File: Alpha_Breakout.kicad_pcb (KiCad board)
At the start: 4 copper layers, 66.7 x 74.4 mm, 161 parts, among them IC1 LM66200DRLR, J10 Conn_01x03, J11 Conn_01x03, J12 Conn_01x03, J14 Conn_01x03, J15 Conn_01x03, J16 Conn_01x03, J18 Conn_01x02, J19 Conn_01x02, J2 USB_C_Receptacle_USB2.0_16P, J20 Conn_01x02, J21 Conn_01x02, J22 Conn_01x02, J23 Conn_01x02, J24 Conn_01x04, J25 Conn_01x02, J26 Conn_01x02, J27 Conn_01x02, J28 Conn_01x02, J29 Conn_01x02, J3 Conn_01x03, J30 Conn_01x04, J31 Conn_01x02, J33 Conn_01x02, J34 Conn_01x02, J35 Conn_02x06_Odd_Even, J36 Conn_01x02, J4 Conn_01x03, J5 Conn_01x03, J7 Conn_01x03, J8 Conn_01x03, J9 Conn_01x03, Q1 CSD13381F4, Q2 CSD13381F4, Q3 CSD13381F4, Q4 CSD13381F4, Q5 SSM3J328R, Q6 L2N7002SLLT1G, SW1 SW_Push, SW2 SW_Push, U1 STM32F103C8Tx, U10 LP2985-3.3, U11 SP3485EN, U12 ADS1231ID, U13 TCA9517ADGK, U2 CH340N, U3 ADS7828, U4 ADS7828, U5 MAX31856, U6 MAX31856, U7 MAX31856, U8 MAX31856, U9 AP63203WU

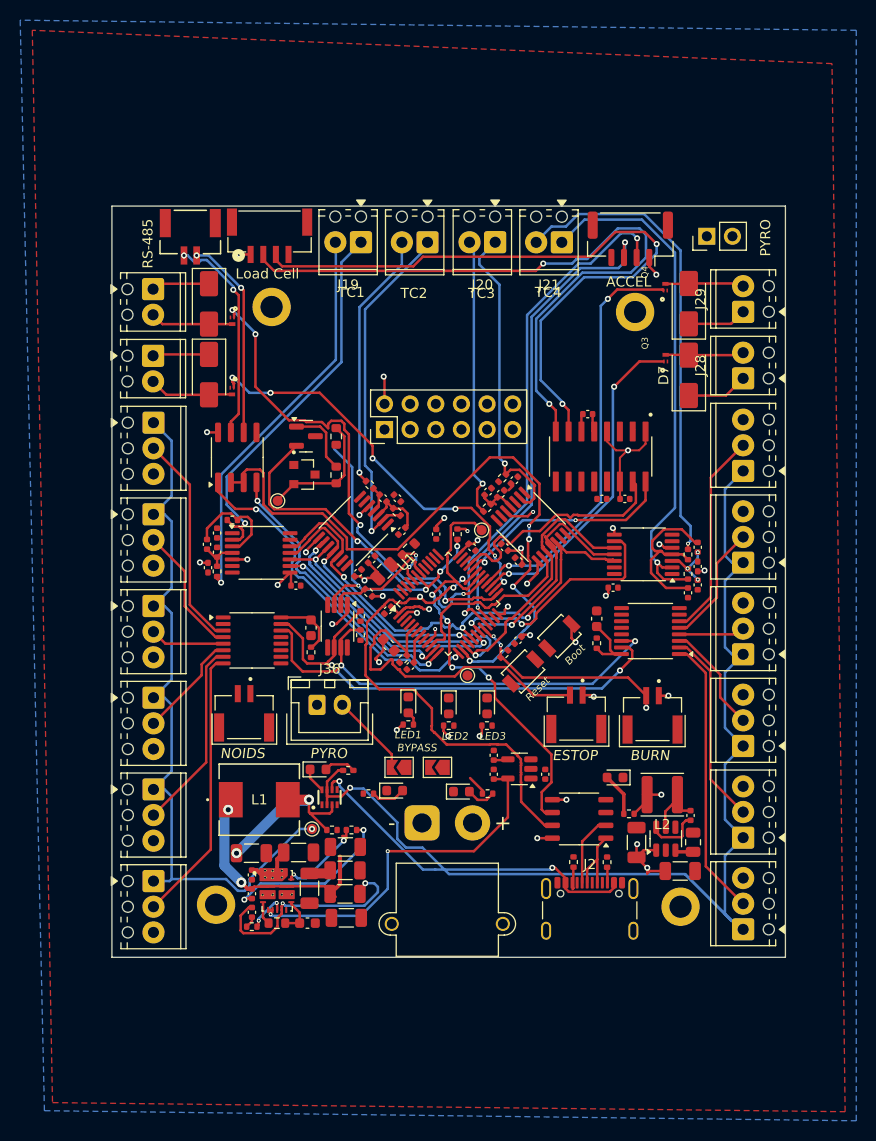
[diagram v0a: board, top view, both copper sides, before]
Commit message: ⚡️⚙️🐘😂
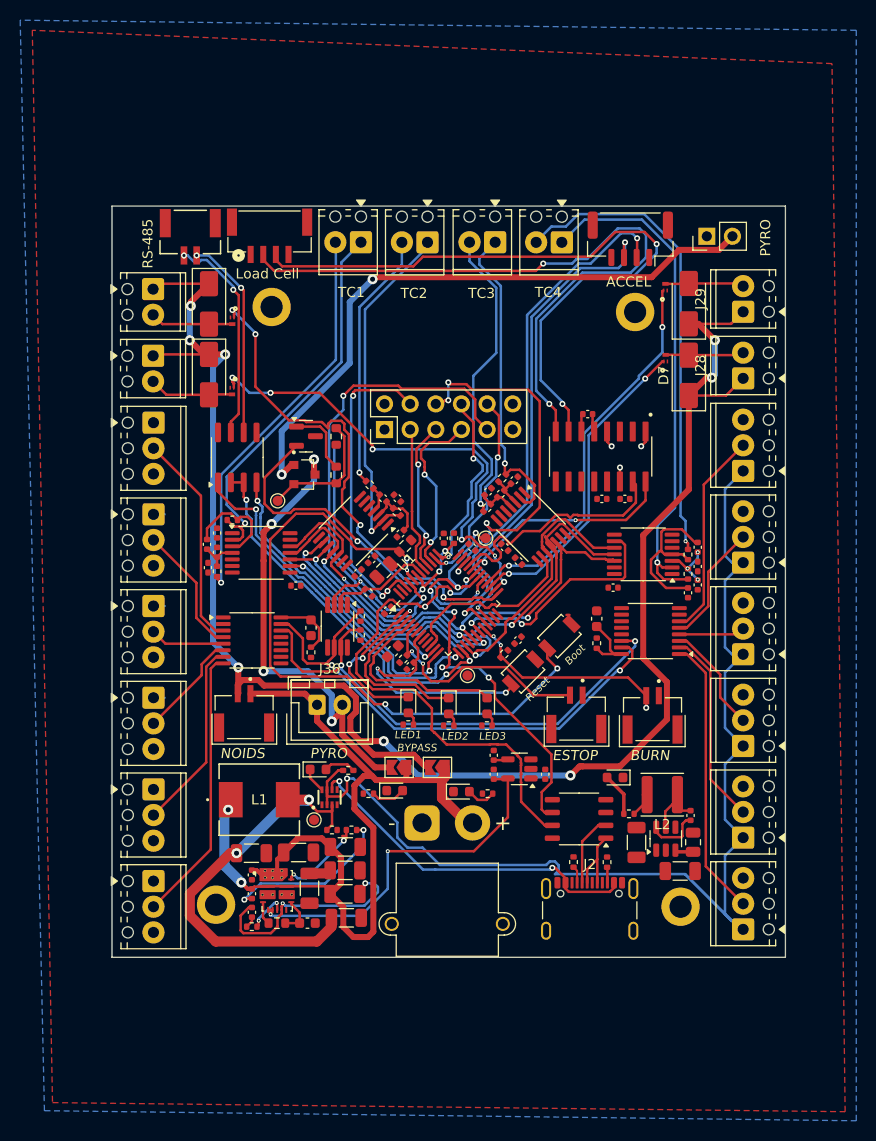
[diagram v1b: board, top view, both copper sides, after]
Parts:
- moved TP4 0.92 mm to (135.1, 123.1)
- moved TP1 0.89 mm to (152.1, 95.2)
- moved C2 0.85 mm to (147.9, 95.2)
- moved C7 0.73 mm to (142.9, 106.4), turned to 45 degrees
- moved R2 0.54 mm to (148.9, 95.2)
- moved R3 0.49 mm to (144.1, 96.0)
- moved C12 0.28 mm to (143.7, 94.7)
- moved C5 0.11 mm to (142.0, 98.4)
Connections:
- J22 pad 1: +BATT -> GND
- J22 pad 2: GND -> +BATT
- J35 pad 3: /Breakout/PB3 -> /Breakout/PB5
- J35 pad 7: /Breakout/PB5 -> /Breakout/PB3
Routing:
- net SW_PWR: track 23.5 -> 174.6 mm, vias 0 -> 8
- net +3.3V: track 85.8 -> 7.88 mm, vias 38 -> 3
- net +5V: track 189.6 -> 120.5 mm, vias 3 -> 1
- net +BATT: track 6.20 -> 71.9 mm
- net Net-(J34-Pin_2): track 0.00 -> 62.1 mm, vias 0 -> 2
- net Net-(U1-BOOT0): track 4.39 -> 66.3 mm, vias 2 -> 4
- net /Breakout/PB8: track 0.00 -> 49.3 mm, vias 0 -> 2
- net /Breakout/PA13: track 0.00 -> 37.6 mm, vias 0 -> 4
- net PYRO_PWR: track 8.23 -> 45.7 mm, vias 0 -> 4
- net /Breakout/PB9: track 0.00 -> 31.1 mm, vias 0 -> 3
- net /RS-485/DIR_RS485: track 67.8 -> 38.1 mm, vias 4 -> 3
- net BATT_V+: track 20.8 -> 45.6 mm
- net Net-(U1-NRST): track 2.97 -> 23.6 mm, vias 0 -> 2
- net /Breakout/PA15: track 0.00 -> 20.3 mm, vias 0 -> 2
- net Net-(D11-K): track 0.00 -> 19.4 mm
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- added copper zone on In2.Cu, net +5V

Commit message: Routed Ground, except for one pad
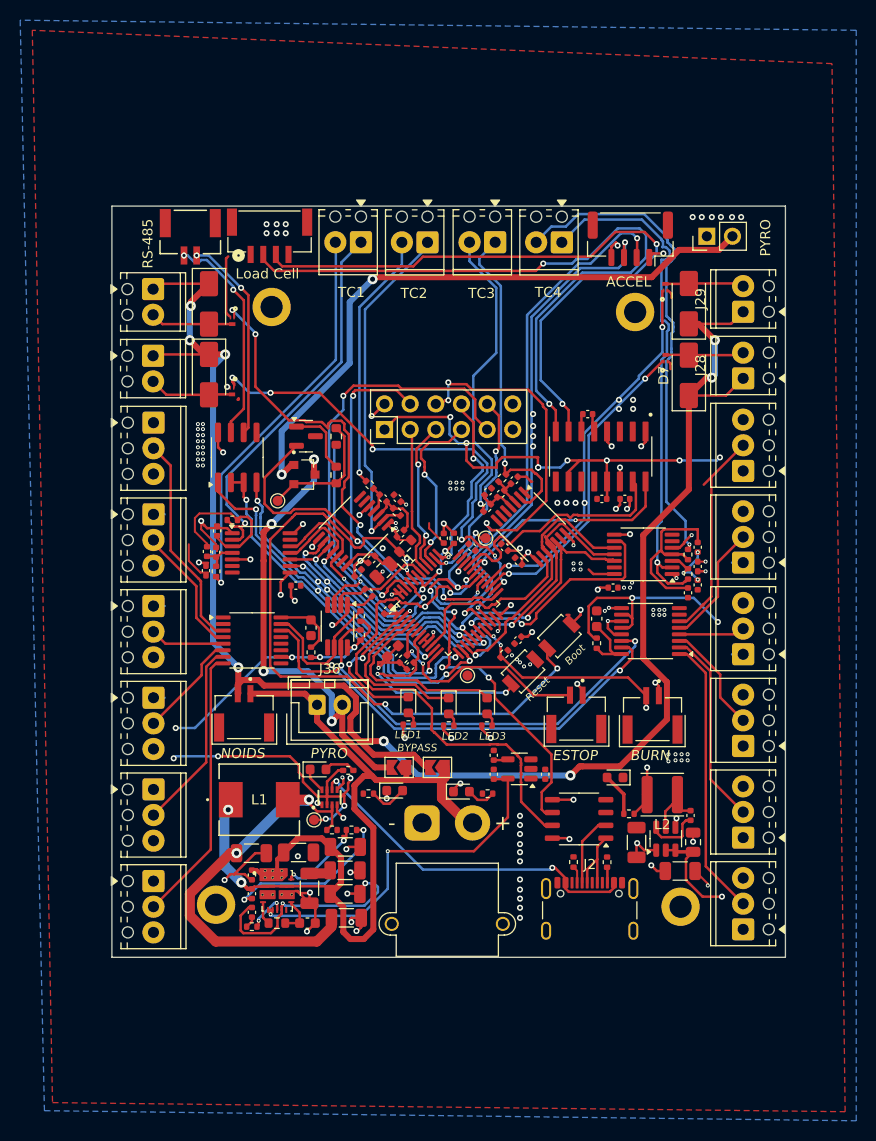
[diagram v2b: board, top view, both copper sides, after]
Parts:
- moved C15 0.71 mm to (124.5, 96.5)
- moved C17 0.36 mm to (124.4, 98.4)
- moved C13 0.21 mm to (125.5, 94.5)
- moved R8 0.10 mm to (125.4, 98.5)
- moved C11 0.10 mm to (125.4, 96.6)
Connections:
- C16 pad 2: +3.3V -> GND
- C17 pad 2: +3.3V -> GND
- C18 pad 1: +3.3V -> GND
- C19 pad 1: +3.3V -> GND
- C2 pad 1: +3.3V -> GND
- C26 pad 2: +3.3V -> GND
- C27 pad 2: +3.3V -> GND
- C28 pad 1: +3.3V -> GND
- C29 pad 1: +3.3V -> GND
- C3 pad 1: +3.3V -> GND
- C30 pad 1: FB -> GND
- C36 pad 1: +3.3V -> GND
- C41 pad 1: +3.3V -> GND
- C5 pad 1: +3.3V -> GND
- C50 pad 2: +3.3V -> GND
- C6 pad 1: +3.3V -> GND
- C7 pad 1: +3.3V -> GND
- J24 pad 1: +3.3V -> GND
- J24 pad 3: /Accelerometer/ACC_SCL -> GND
- J31 pad 1: +3.3V -> GND
- J33 pad 1: +3.3V -> GND
- J35 pad 2: +3.3V -> GND
- L2 pad 2: +3.3V -> GND
- PS1 pad 8: FB -> GND
- Q3 pad 1: /Solenoids/S3 -> GND
- Q4 pad 1: /Solenoids/S4 -> GND
- R1 pad 1: +3.3V -> GND
- R18 pad 1: +3.3V -> GND
- R2 pad 1: +3.3V -> GND
- R28 pad 1: +3.3V -> GND
- R29 pad 1: +3.3V -> GND
- R30 pad 1: +3.3V -> GND
- SW2 pad 1: +3.3V -> GND
- U1 pad 1: +3.3V -> GND
- U1 pad 11: /stm32f1/TC3_CS -> GND
- U1 pad 12: /RS-485/TX_RS485 -> GND
- U1 pad 13: /RS-485/RX_RS485 -> GND
- U1 pad 15: /stm32f1/SPI1_SCK -> GND
- U1 pad 18: /stm32f1/TC1_CS -> GND
- U1 pad 22: /Accelerometer/ACC_SCL -> GND
- U1 pad 24: +3.3V -> GND
- U1 pad 27: /Solenoids/S3 -> GND
- U1 pad 28: /Solenoids/S4 -> GND
- U1 pad 48: +3.3V -> GND
- U1 pad 9: +3.3V -> GND
- U11 pad 1: /RS-485/RX_RS485 -> GND
- U11 pad 4: /RS-485/TX_RS485 -> GND
- U11 pad 8: +3.3V -> GND
- U12 pad 1: +3.3V -> GND
- U12 pad 14: +3.3V -> GND
- U12 pad 4: +3.3V -> GND
- U13 pad 1: +3.3V -> GND
- U2 pad 5: +3.3V -> GND
- U2 pad 8: +3.3V -> GND
- U5 pad 10: /stm32f1/SPI1_SCK -> GND
- U5 pad 5: +3.3V -> GND
- U5 pad 8: +3.3V -> GND
- U5 pad 9: /stm32f1/TC1_CS -> GND
- U6 pad 10: /stm32f1/SPI1_SCK -> GND
- U6 pad 5: +3.3V -> GND
- U6 pad 8: +3.3V -> GND
- U6 pad 9: /stm32f1/TC3_CS -> GND
- U7 pad 10: /stm32f1/SPI1_SCK -> GND
- U7 pad 8: +3.3V -> GND
- U8 pad 10: /stm32f1/SPI1_SCK -> GND
- U8 pad 5: +3.3V -> GND
- U8 pad 8: +3.3V -> GND
- U9 pad 1: +3.3V -> GND
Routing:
- net GND: track 0.04 -> 476.7 mm, vias 0 -> 178
- net /stm32f1/SPI1_SCK: track 55.4 -> 0.00 mm, vias 2 -> 0
- net /Accelerometer/ACC_SCL: track 48.9 -> 0.00 mm, vias 2 -> 0
- net /Solenoids/S4: track 38.2 -> 0.00 mm, vias 2 -> 0
- net /RS-485/RX_RS485: track 36.7 -> 0.00 mm, vias 2 -> 0
- net /Solenoids/S3: track 31.3 -> 0.00 mm, vias 2 -> 0
- net /RS-485/TX_RS485: track 31.1 -> 0.00 mm, vias 2 -> 0
- net /stm32f1/TC1_CS: track 26.1 -> 0.00 mm, vias 2 -> 0
- net +5V: track 120.5 -> 144.2 mm, vias 1 -> 20
- net FB: track 21.5 -> 0.00 mm, vias 2 -> 0
- net /stm32f1/TC3_CS: track 18.3 -> 0.00 mm, vias 2 -> 0
- net +3.3V: track 7.88 -> 0.00 mm, vias 3 -> 0
- net Net-(U6-T-): track 10.4 -> 15.3 mm
- net Net-(J21-Pin_2): track 46.9 -> 48.4 mm
- net Net-(U8-T-): track 5.50 -> 6.92 mm
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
